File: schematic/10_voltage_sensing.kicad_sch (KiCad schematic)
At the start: 30 parts, among them U801 TLV9064IPWR

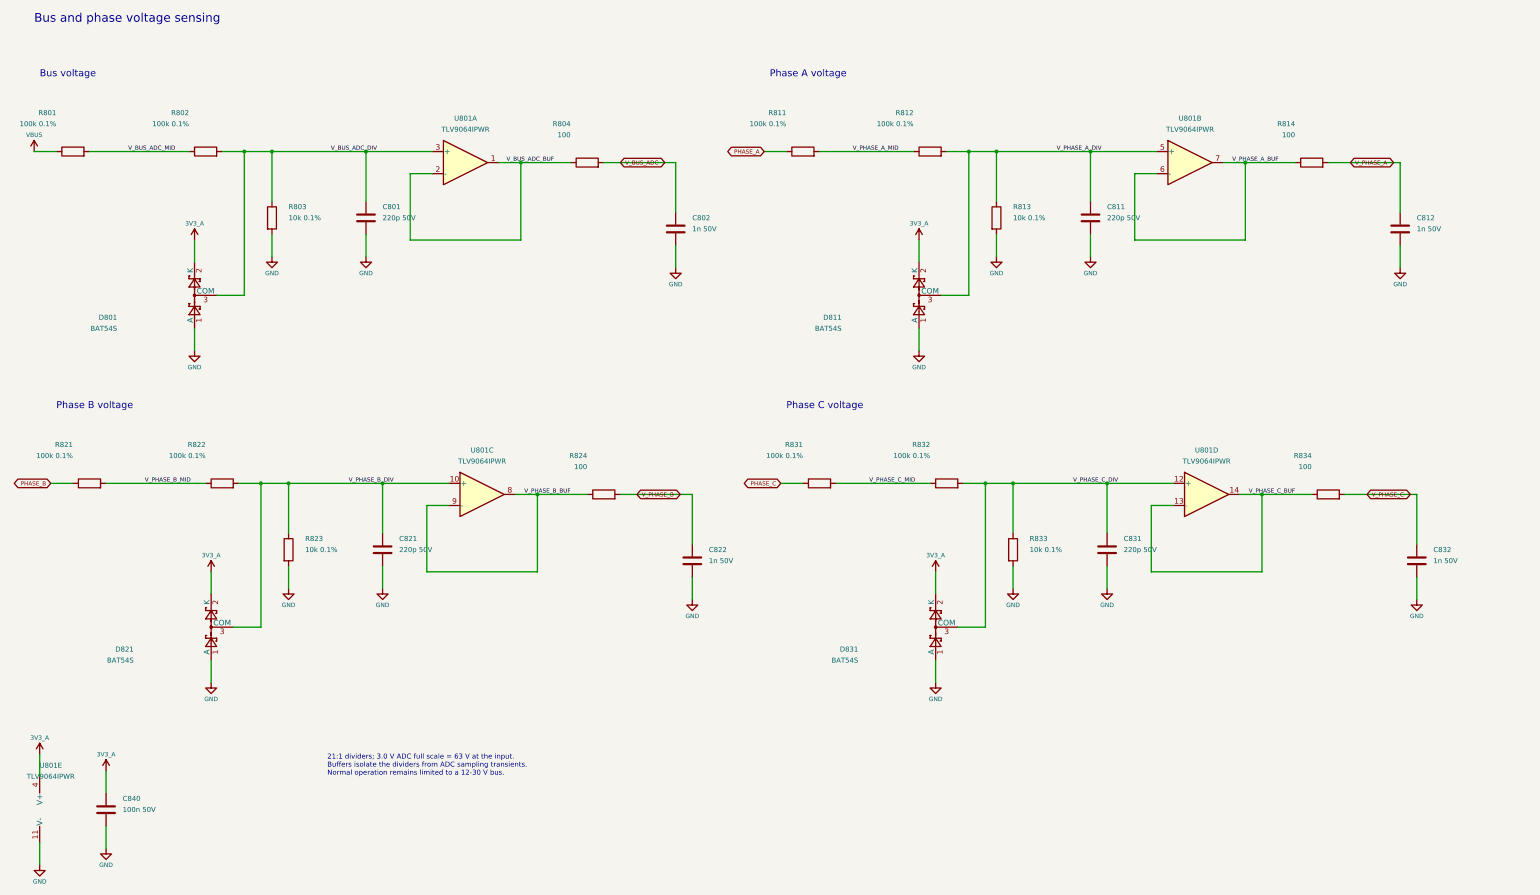
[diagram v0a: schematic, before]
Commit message: devlog 03
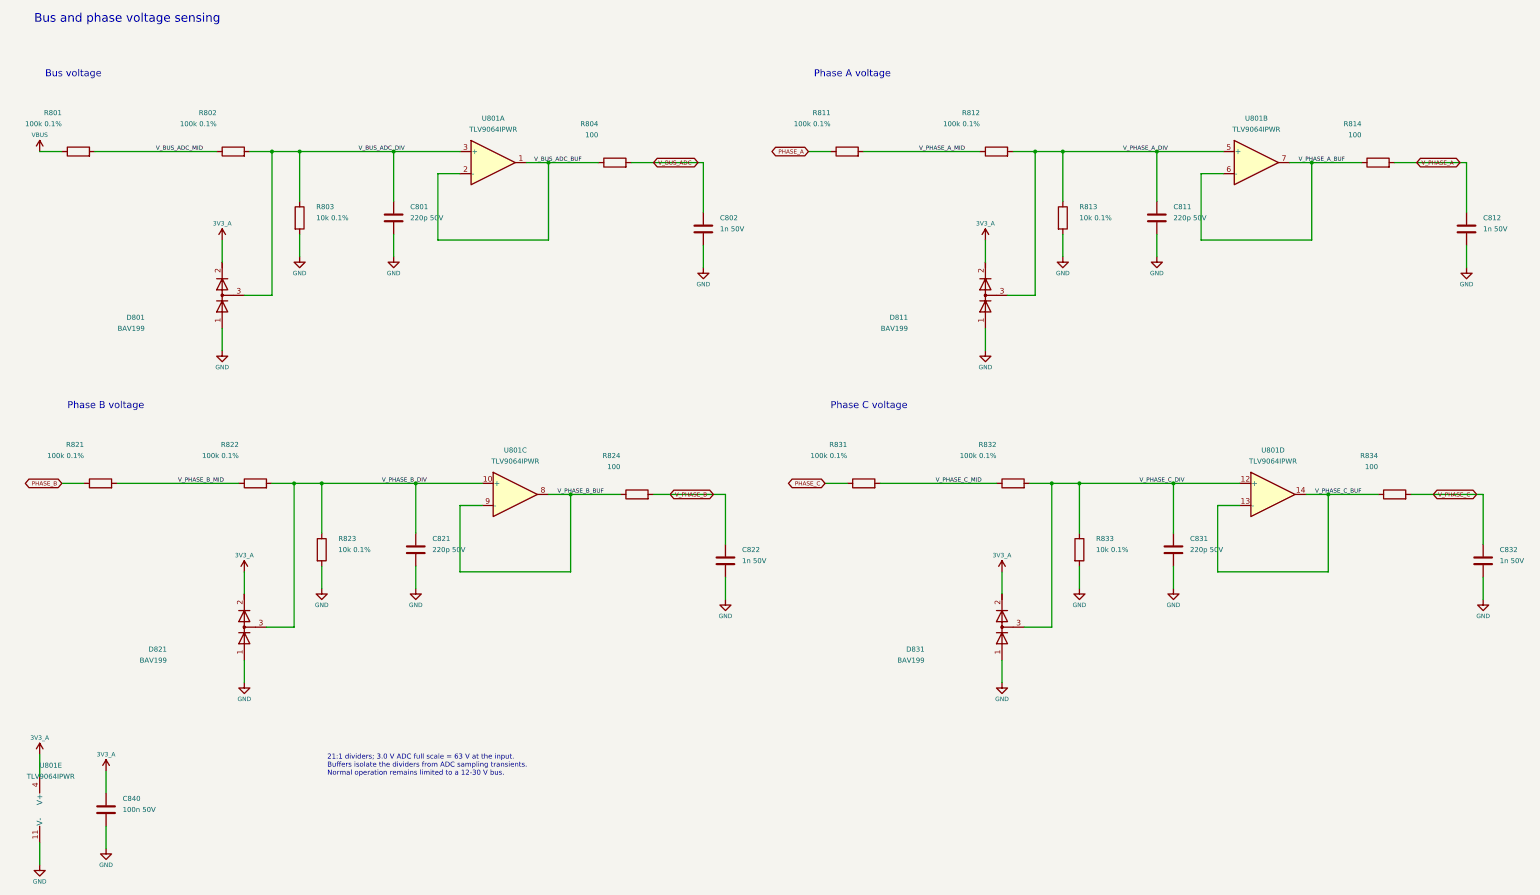
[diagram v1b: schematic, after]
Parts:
- D801, D811, D821, D831: value BAT54S -> BAV199; symbol Diode:BAT54S -> Device:D_Dual_Series_AKC; MPN BAT54S,215 -> BAV199,215
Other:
- moved on the sheet: C801, C802, C811, C812, C821, C822, C831, C832, R801, R802, R803, R804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
